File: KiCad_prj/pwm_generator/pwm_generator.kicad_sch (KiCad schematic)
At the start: 18 parts, among them J1 MLW20A, J2 MLW10A, U1 LM2664 / LM2665, U2 74HC14, U3 TL431DBV

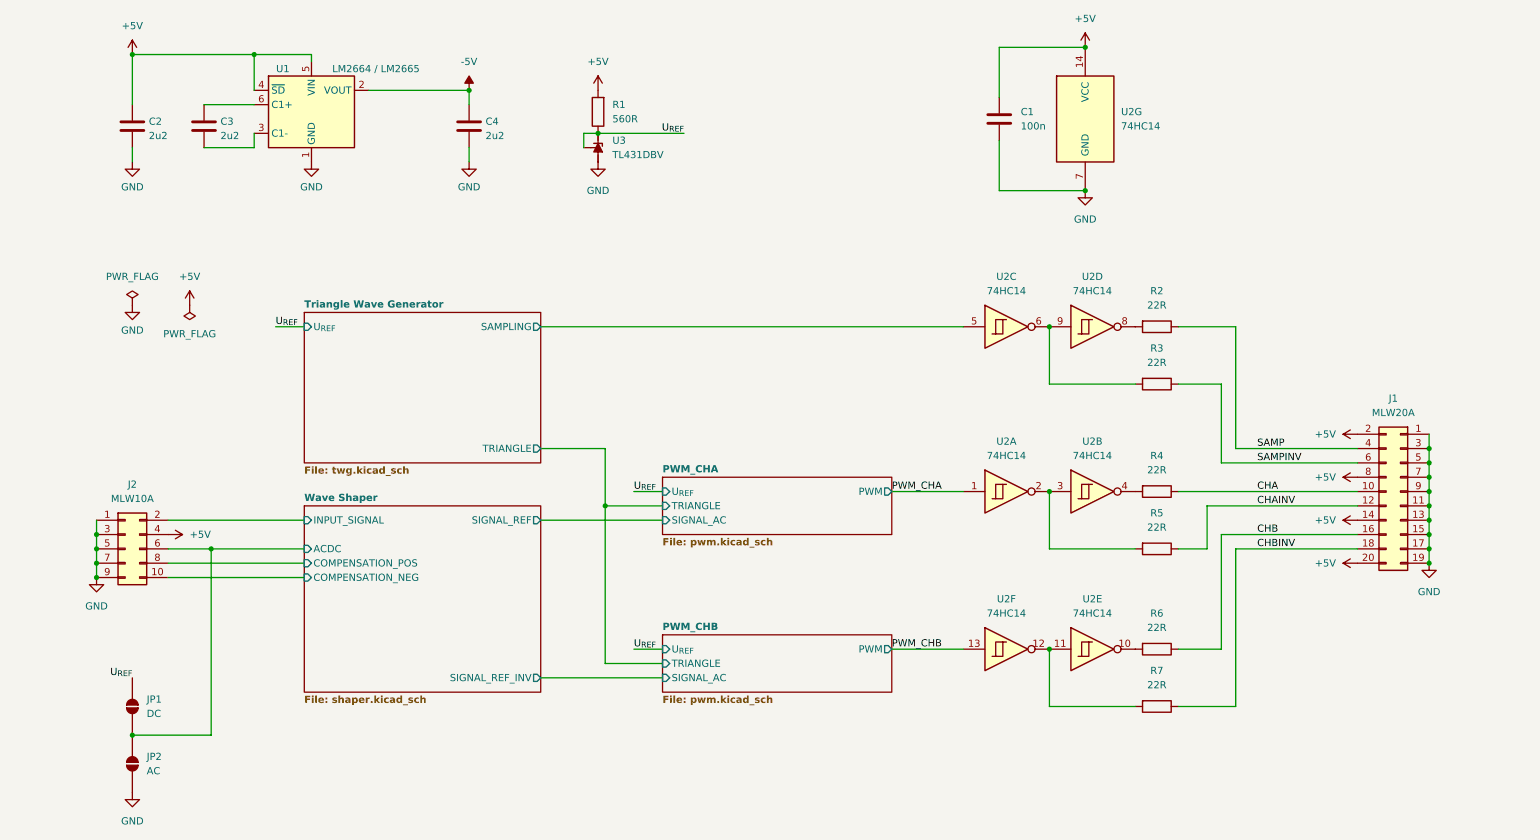
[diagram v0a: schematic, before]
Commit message: Pocatek prace na DPS
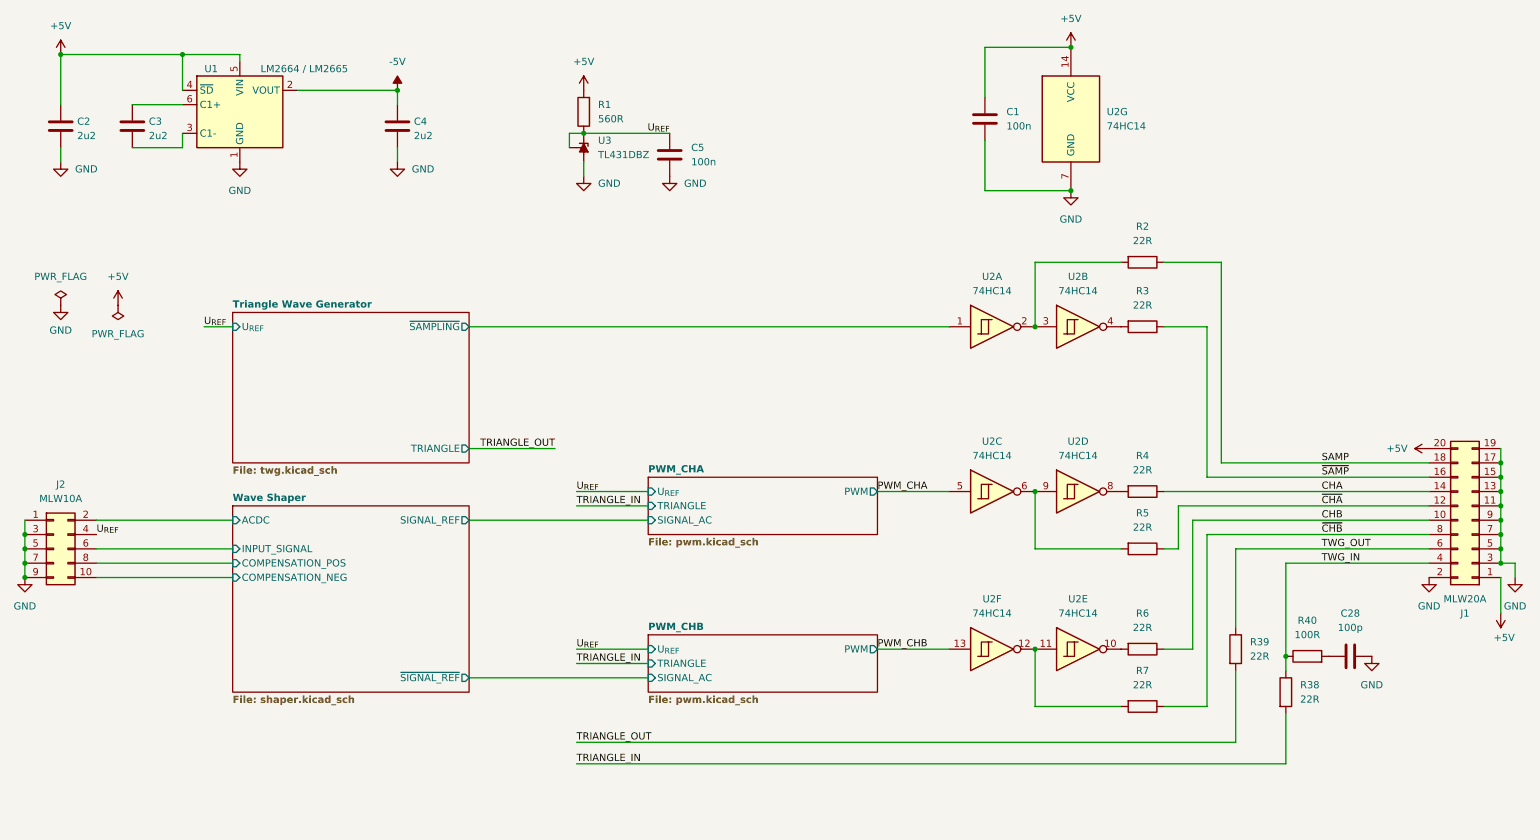
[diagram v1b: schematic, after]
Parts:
- removed JP1: DC, Jumper:SolderJumper-2_P1.3mm_Open_RoundedPad1.0x1.5mm, symbol Jumper:SolderJumper_2_Open
- removed JP2: AC, Jumper:SolderJumper-2_P1.3mm_Open_RoundedPad1.0x1.5mm, symbol Jumper:SolderJumper_2_Open
- removed U3: TL431DBV, Package_TO_SOT_SMD:SOT-23-5, symbol Reference_Voltage:TL431DBV
- added C28: 100p, Capacitor_SMD:C_0805_2012Metric, symbol Device:C
- added C5: 100n, Capacitor_SMD:C_0805_2012Metric, symbol Device:C
- added R38, R39: 22R, Resistor_SMD:R_0805_2012Metric, symbol Device:R
- added R40: 100R, Resistor_SMD:R_0805_2012Metric, symbol Device:R
- added U3: TL431DBZ, Package_TO_SOT_SMD:SOT-23, symbol Reference_Voltage:TL431DBZ
- renumbered R5 to R4, R4 to R5, R7 to R6, R6 to R7
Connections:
- net Triangle Wave Generator/SAMPLING is gone; now on net PWM_CHA: U2.5
- net +5V: now also J1.1 (Pin_1); no longer J1.14 (Pin_14), J1.2 (Pin_2), J1.8 (Pin_8), J2.4 (Pin_4)
- net CHA: now also J1.14 (Pin_14), R4.1; no longer J1.10 (Pin_10), R5.1
- net CHB: now also J1.10 (Pin_10), R6.1; no longer J1.16 (Pin_16), R7.1
- net GND: now also J1.2 (Pin_2), C28.2, C5.1, U3.3 (A); no longer J1.1 (Pin_1)
- net PWM_CHA: no longer U2.1
- net SAMP: now also J1.18 (Pin_18); no longer J1.4 (Pin_4)
- net U_{REF}: now also J2.4 (Pin_4), C5.2, U3.1 (K), U3.2 (REF)
- net Wave Shaper/ACDC: now also J2.2 (Pin_2); no longer J2.6 (Pin_6)
- net Wave Shaper/INPUT_SIGNAL: now also J2.6 (Pin_6); no longer J2.2 (Pin_2)
- net at R7.2: now also U2.11, U2.12; no longer U2.10
- net at U2.8: now also R4.2; no longer R2.2
- net at U2.6, U2.9: now also R5.2; no longer R3.2
- net at U2.2, U2.3: now also R2.2; no longer R4.2
- net at U2.4: now also R3.2; no longer R5.2
- net CHAINV renamed ~{CHA}
- net ~{CHA}: now also R5.1; no longer R4.1
- removed net CHBINV: J1.18 (Pin_18), R6.1
- net SAMPINV renamed TWG_OUT
- net TWG_OUT: now also R39.1; no longer R3.1
- new net: R6.2, U2.10
- new net: C28.1, R40.2
- new net TRIANGLE_IN: R38.2
- new net TRIANGLE_OUT: R39.2
- new net TWG_IN: J1.4 (Pin_4), R38.1, R40.1
- new net Triangle Wave Generator/~{SAMPLING}: U2.1
- new net ~{CHB}: J1.8 (Pin_8), R7.1
- new net ~{SAMP}: J1.16 (Pin_16), R3.1
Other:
- sheet Triangle Wave Generator ports: added ~{SAMPLING}; removed SAMPLING
- sheet Wave Shaper ports: added ~{SIGNAL_REF}; removed SIGNAL_REF_INV
- moved on the sheet: C1, C2, C3, C4, J1, J2, R1, R2, R3, R4, R5, R6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
